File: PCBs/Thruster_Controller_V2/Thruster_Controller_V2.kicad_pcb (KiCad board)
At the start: 4 copper layers, 35.5 x 37 mm, 112 parts, among them J1 PHASE_A, J2 PHASE_B, J3 PHASE_C, J4 Conn_01x01, J5 Pogo Conn, J6 Conn_01x01, J7 Conn_01x01, J8 Conn_01x01, Q1 SIZF906DT, Q2 SIZF906DT, Q3 SIZF906DT, U1 NCP718AMT330, U2 TMS320F280041C, U3 DRV8320S, U4 NCP718BMT500, U8 ATA6561, Y1 20 MHz

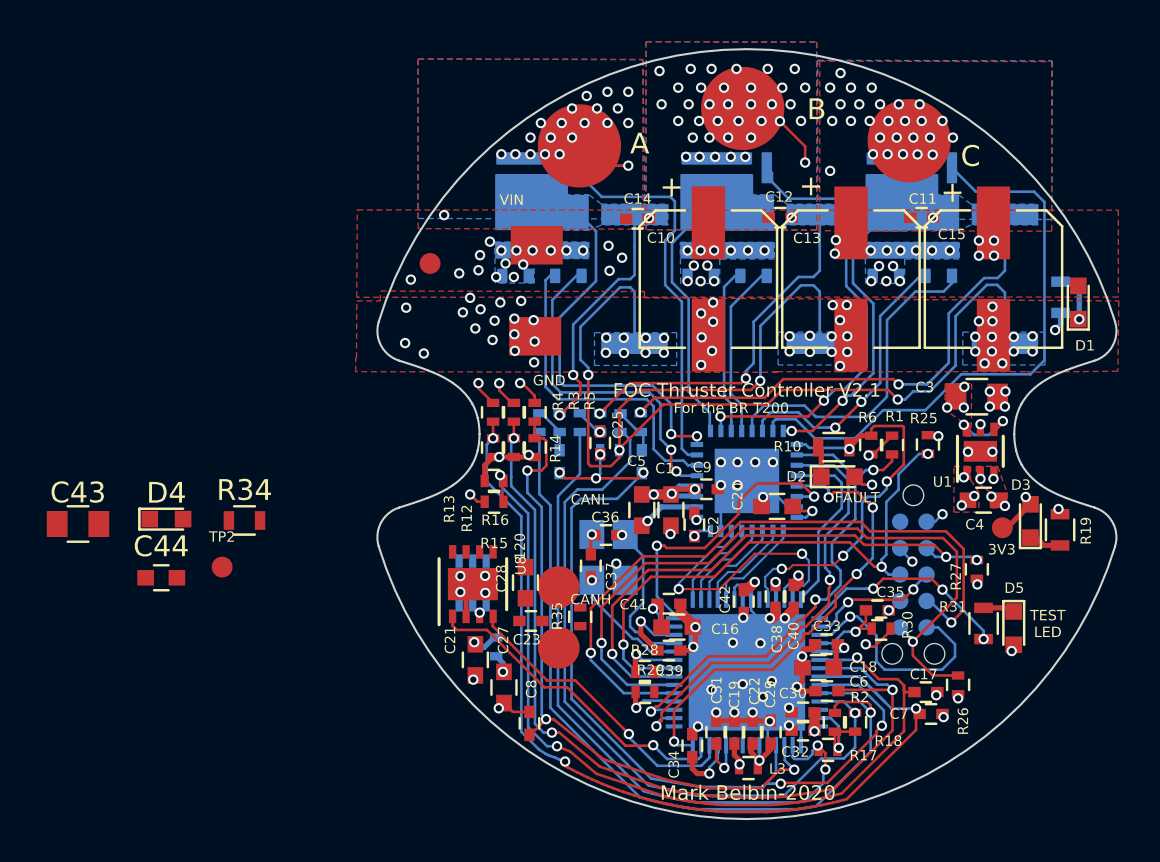
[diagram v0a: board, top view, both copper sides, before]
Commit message: Routing and Layout
- Finished layout
- Finished routing
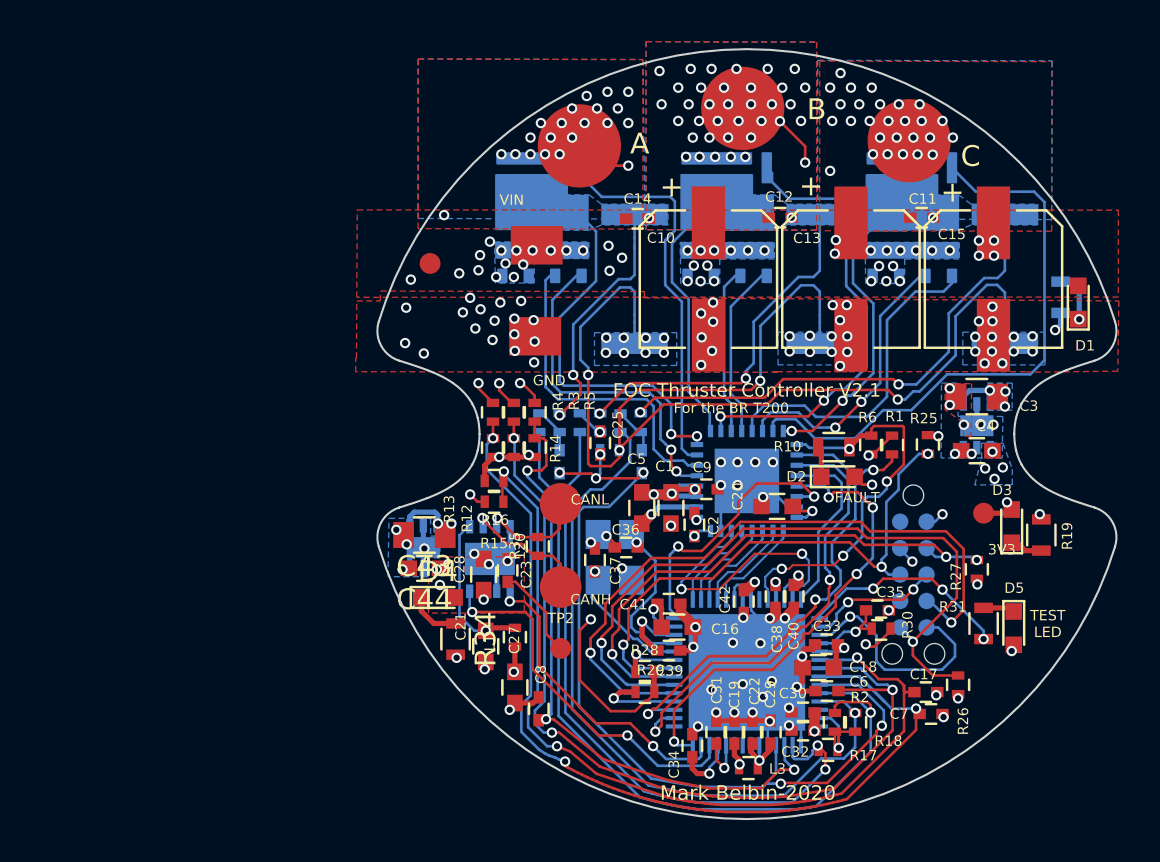
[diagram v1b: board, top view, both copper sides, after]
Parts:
- L1: moved to F.Cu
- U1, U8: moved to B.Cu
- moved TP2 16.7 mm to (91.0, 108.5)
- moved C43 16.7 mm to (84.5, 103.1), turned to 180 degrees
- moved D4 13.6 mm to (85.2, 106.1)
- moved C44 12.7 mm to (84.5, 104.7), turned to 180 degrees
- moved R34 11.6 mm to (86.0, 108.1), turned to 270 degrees
- moved J6 4.00 mm to (91.0, 101.6)
- moved R35 3.95 mm to (90.0, 103.7)
- moved J4 2.92 mm to (91.0, 105.6)
- moved U4 2.92 mm to (84.5, 103.7)
- moved C23 2.68 mm to (88.5, 104.8), turned to 90 degrees
- moved C4 2.40 mm to (111.0, 99.0), turned to 180 degrees
- moved C28 2.05 mm to (87.3, 105.0)
- moved U8 1.46 mm to (87.7, 104.2)
- moved U1 1.24 mm to (111.0, 97.8)
- moved C36 1.14 mm to (94.2, 103.7)
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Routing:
- net +3V3: track 11.4 -> 25.9 mm, vias 14 -> 16
- net GND: track 40.6 -> 49.5 mm, vias 111 -> 112
- net /CANL: track 0.00 -> 6.25 mm, vias 0 -> 1
- net /CANH: track 0.00 -> 5.19 mm, vias 0 -> 1
- net +5V: track 0.18 -> 5.06 mm, vias 1 -> 4
- net /RXCAN: track 14.4 -> 17.7 mm, vias 1 -> 2
- net Net-(D4-Pad1): track 0.00 -> 2.55 mm
- net +BATT: track 11.0 -> 12.9 mm
- net /TI_MCU/GPIO24: track 2.76 -> 4.14 mm
- net /Powertrain/EN_GATE: track 14.2 -> 13.1 mm
- net /Powertrain/VSEN_PVDD: track 41.7 -> 42.6 mm
- net /TXCAN: track 15.7 -> 14.9 mm, vias 1 -> 2
- net /Powertrain/ISEN_C: track 35.6 -> 34.9 mm
- net /Powertrain/ISEN_B: track 32.6 -> 32.0 mm
- net /Powertrain/PGA_GND: track 43.5 -> 42.9 mm
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- added copper zone on B.Cu, net +3V3
- added copper zone on F.Cu, net +5V
- removed copper zone on F.Cu, net +3V3
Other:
- rule trace_min: 0.0889 -> 0
